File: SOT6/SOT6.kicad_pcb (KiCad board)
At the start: 2 copper layers, 8.9 x 11.4 mm, 5 parts, among them J1 Conn_01x03, J2 Conn_01x03, J3 Conn_02x03_Counter_Clockwise, J4 Conn_02x03_Counter_Clockwise

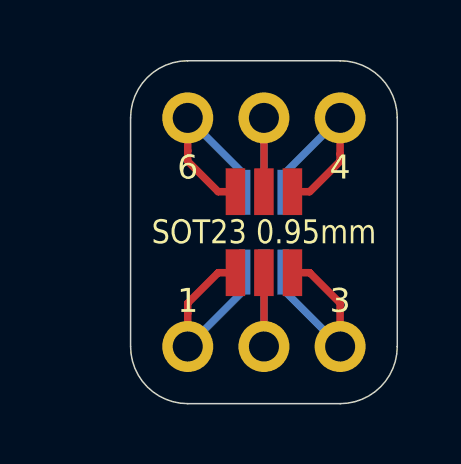
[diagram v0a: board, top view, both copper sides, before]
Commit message: Board Updates
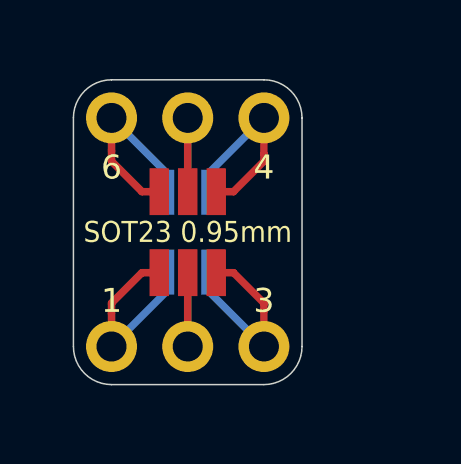
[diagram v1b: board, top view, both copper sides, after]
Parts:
- moved J3 2.54 mm to (65.5, 36.8)
- moved J4 2.54 mm to (65.5, 36.8)
- moved J1 2.54 mm to (63.0, 33.0)
- moved J2 2.54 mm to (63.0, 40.6)
- moved G*** 2.29 mm to (63.0, 36.8)
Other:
- board size 8.9 x 11.4 mm -> 7.6 x 10.2 mm
